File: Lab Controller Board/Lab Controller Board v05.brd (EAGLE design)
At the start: 50 x 50 mm, 48 parts, among them Q2 MMBT5088, Q3 100A/100V, Q4 MMBT5088, Q5 100A/100V, Q6 MMBT5088, Q7 100A/100V, Q8 MMBT5088, U1 ATMEGA328P_TQFP, U2 CH340G, Y1 16MHZ

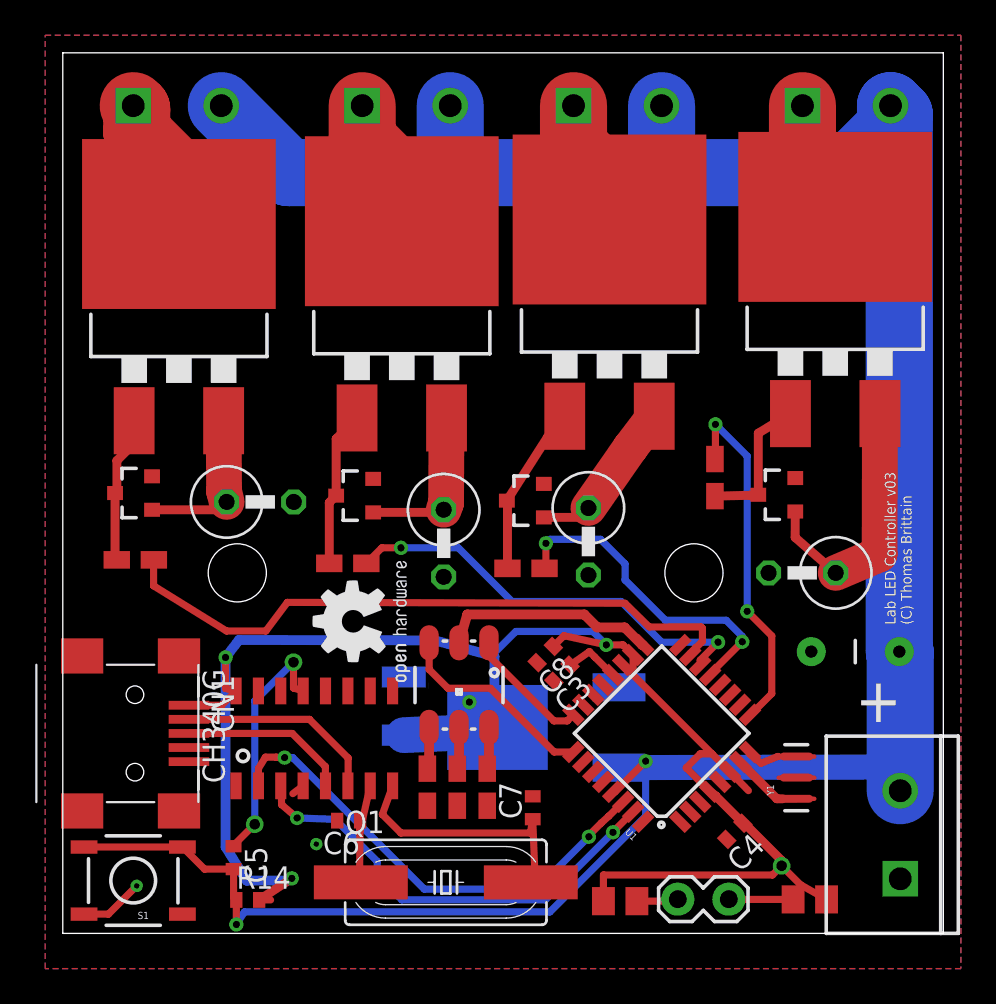
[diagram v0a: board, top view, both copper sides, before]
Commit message: Hmm
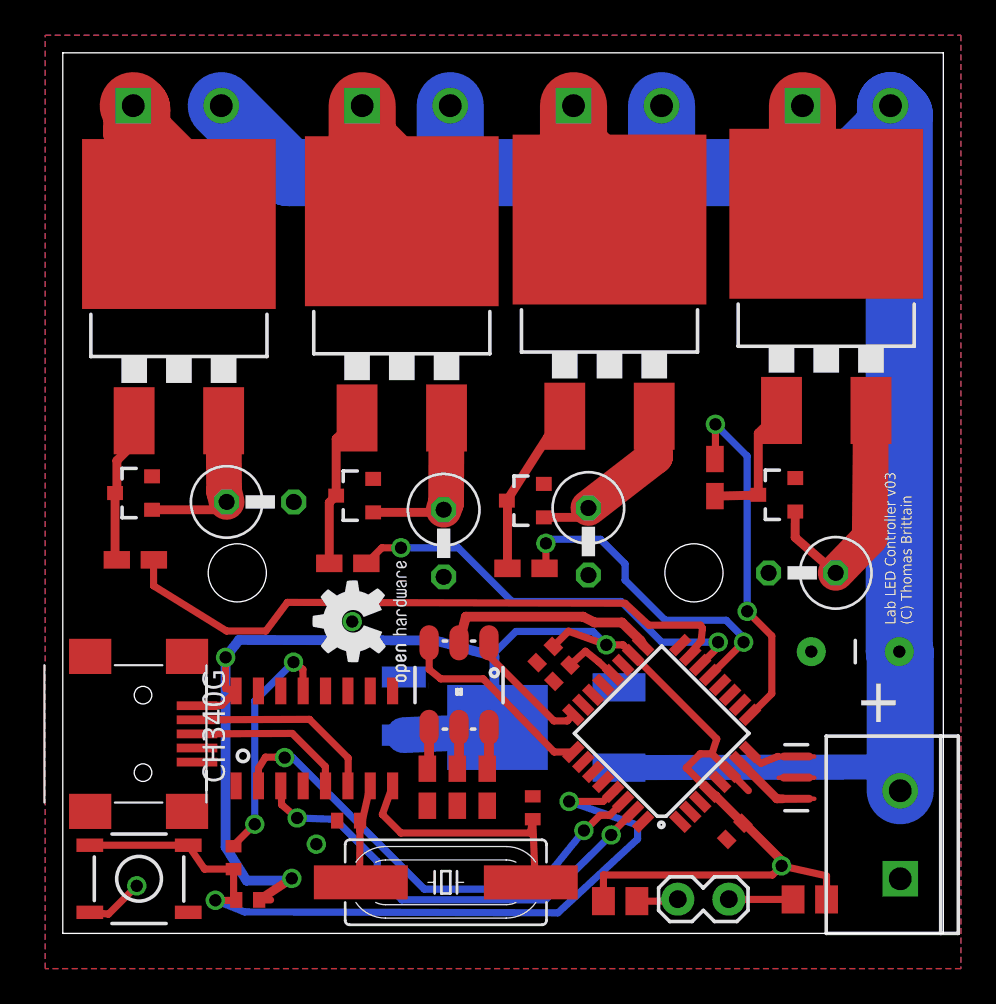
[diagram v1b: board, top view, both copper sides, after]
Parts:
- moved Q5 0.54 mm to (43.4, 36.7)
- moved CN1 0.46 mm to (3.56, 11.3)
- moved S1 0.35 mm to (4.33, 3.10)
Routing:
- net N$13: track 43.8 -> 45.4 mm
- net N$32: track 0.73 -> 0.00 mm
- net FET_SOURCE2: track 15.2 -> 14.5 mm
- net FET_SOURCE3: track 9.21 -> 9.86 mm
- net VCC: track 97.7 -> 98.4 mm
